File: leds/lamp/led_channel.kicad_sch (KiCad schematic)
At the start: 12 parts, among them J2 Conn_02x05_Top_Bottom, U19 MP5048AGU-Z

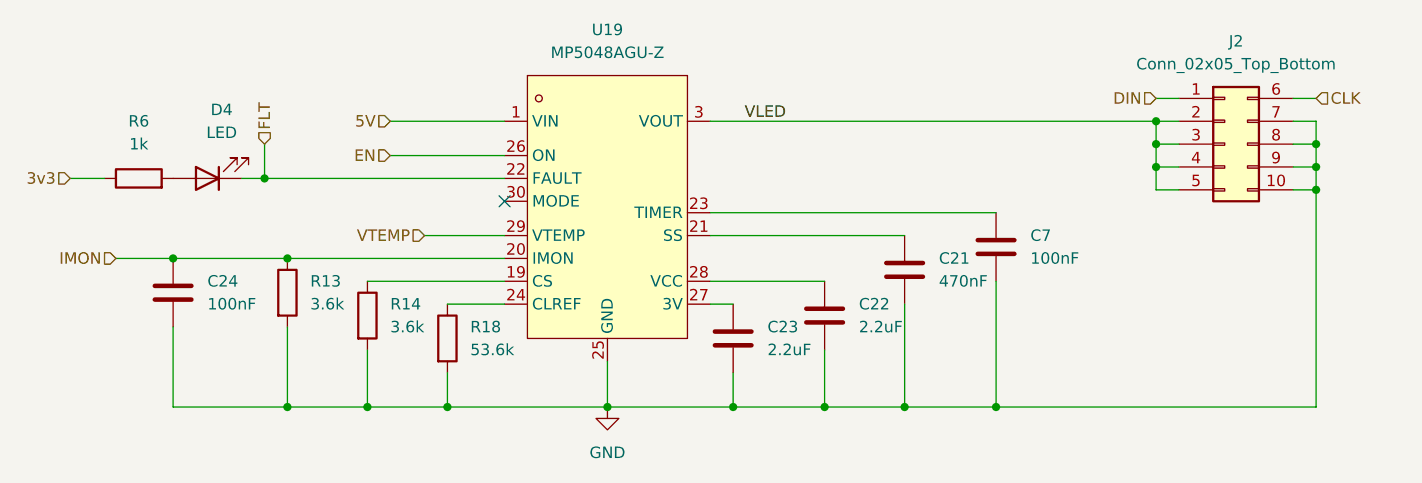
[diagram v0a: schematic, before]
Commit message: WIP: Lamp
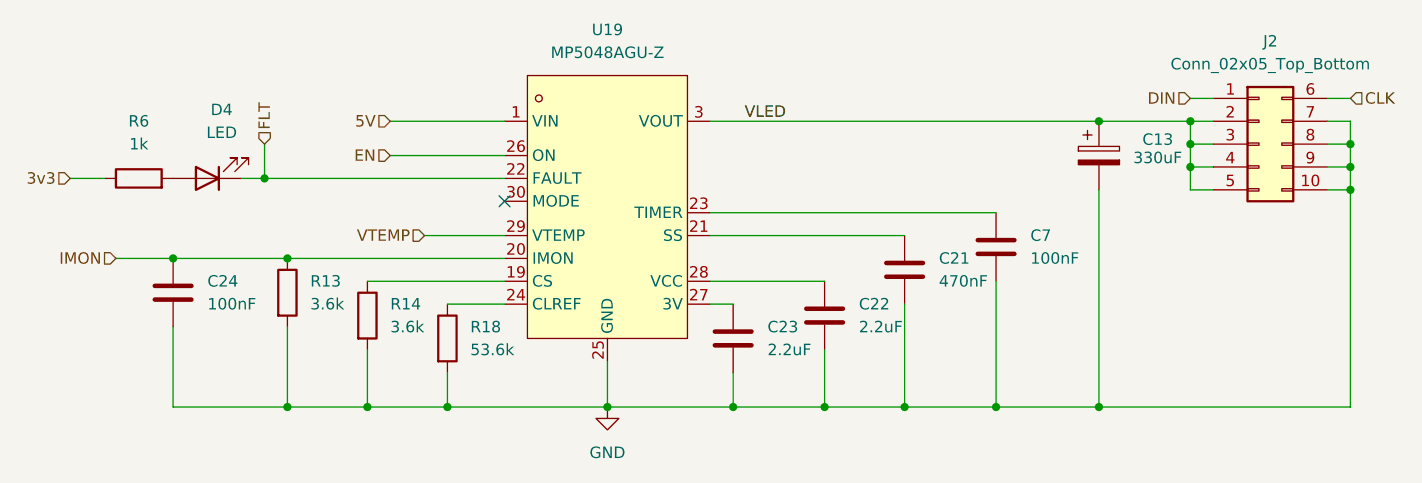
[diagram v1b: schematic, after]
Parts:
- added C13: 330uF, easyeda2kicad:CAP-SMD_L7.3-W4.3-FD, symbol Device:C_Polarized
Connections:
- net GND: now also C13.2
- net VLED: now also C13.1
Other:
- moved on the sheet: J2
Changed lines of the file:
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@@
 	)
 	(junction
-		(at 264.16 74.93)
+		(at 267.97 74.93)
 		(diameter 0)
 		(color 0 0 0 0)
@@
 	)
 	(junction
-		(at 246.38 69.85)
+		(at 250.19 69.85)
 		(diameter 0)
 		(color 0 0 0 0)
@@
 	)
 	(junction
-		(at 246.38 74.93)
+		(at 250.19 74.93)
 		(diameter 0)
 		(color 0 0 0 0)
@@
 	)
 	(junction
-		(at 264.16 72.39)
+		(at 267.97 72.39)
+		(diameter 0)
+		(color 0 0 0 0)
+	)
+	(junction
+		(at 240.03 101.6)
 		(diameter 0)
 		(color 0 0 0 0)
@@
 	)
 	(junction
-		(at 264.16 77.47)
+		(at 267.97 77.47)
 		(diameter 0)
 		(color 0 0 0 0)
@@
 	)
 	(junction
-		(at 246.38 72.39)
+		(at 240.03 69.85)
+		(diameter 0)
+		(color 0 0 0 0)
+	)
+	(junction
+		(at 250.19 72.39)
 		(diameter 0)
 		(color 0 0 0 0)
@@
 	(wire
 		(pts
-			(xy 264.16 74.93) (xy 264.16 77.47)
+			(xy 267.97 74.93) (xy 267.97 77.47)
 		)
 		(stroke
@@
 	(wire
 		(pts
+			(xy 240.03 69.85) (xy 250.19 69.85)
+		)
+		(stroke
+			(width 0)
+			(type default)
+		)
+	)
+	(wire
+		(pts
 			(xy 209.55 101.6) (xy 199.39 101.6)
 		)
@@
 	(wire
 		(pts
-			(xy 264.16 69.85) (xy 264.16 72.39)
+			(xy 267.97 69.85) (xy 267.97 72.39)
 		)
 		(stroke
@@
 	(wire
 		(pts
-			(xy 261.62 67.31) (xy 264.16 67.31)
+			(xy 265.43 67.31) (xy 267.97 67.31)
 		)
 		(stroke
@@
 	(wire
 		(pts
+			(xy 196.85 69.85) (xy 240.03 69.85)
+		)
+		(stroke
+			(width 0)
+			(type default)
+		)
+	)
+	(wire
+		(pts
 			(xy 125.73 76.2) (xy 129.54 76.2)
 		)
@@
 	(wire
 		(pts
+			(xy 240.03 101.6) (xy 267.97 101.6)
+		)
+		(stroke
+			(width 0)
+			(type default)
+		)
+	)
+	(wire
+		(pts
 			(xy 196.85 90.17) (xy 199.39 90.17)
 		)
@@
 	(wire
 		(pts
-			(xy 261.62 72.39) (xy 264.16 72.39)
+			(xy 265.43 72.39) (xy 267.97 72.39)
 		)
 		(stroke
@@
 	(wire
 		(pts
-			(xy 261.62 77.47) (xy 264.16 77.47)
+			(xy 265.43 77.47) (xy 267.97 77.47)
 		)
 		(stroke
@@
 	(wire
 		(pts
-			(xy 248.92 74.93) (xy 246.38 74.93)
+			(xy 252.73 74.93) (xy 250.19 74.93)
 		)
 		(stroke
@@
 	(wire
 		(pts
-			(xy 246.38 77.47) (xy 246.38 74.93)
+			(xy 250.19 77.47) (xy 250.19 74.93)
 		)
 		(stroke
@@
 	(wire
 		(pts
-			(xy 261.62 74.93) (xy 264.16 74.93)
-		)
-		(stroke
-			(width 0)
-			(type default)
-		)
-	)
-	(wire
-		(pts
-			(xy 264.16 77.47) (xy 264.16 101.6)
-		)
-		(stroke
-			(width 0)
-			(type default)
-		)
-	)
-	(wire
-		(pts
-			(xy 264.16 101.6) (xy 228.6 101.6)
-		)
-		(stroke
-			(width 0)
-			(type default)
-		)
-	)
-	(wire
-		(pts
-			(xy 248.92 72.39) (xy 246.38 72.39)
-		)
-		(stroke
-			(width 0)
-			(type default)
-		)
-	)
-	(wire
-		(pts
-			(xy 248.92 77.47) (xy 246.38 77.47)
+			(xy 265.43 74.93) (xy 267.97 74.93)
+		)
+		(stroke
+			(width 0)
+			(type default)
+		)
+	)
+	(wire
+		(pts
+			(xy 267.97 77.47) (xy 267.97 101.6)
+		)
+		(stroke
+			(width 0)
+			(type default)
+		)
+	)
+	(wire
+		(pts
+			(xy 252.73 72.39) (xy 250.19 72.39)
+		)
+		(stroke
+			(width 0)
+			(type default)
+		)
+	)
+	(wire
+		(pts
+			(xy 252.73 77.47) (xy 250.19 77.47)
 		)
 		(stroke
@@
 	(wire
 		(pts
-			(xy 246.38 72.39) (xy 246.38 69.85)
+			(xy 228.6 101.6) (xy 240.03 101.6)
+		)
+		(stroke
+			(width 0)
+			(type default)
+		)
+	)
+	(wire
+		(pts
+			(xy 250.19 72.39) (xy 250.19 69.85)
 		)
 		(stroke
@@
 	(wire
 		(pts
-			(xy 196.85 69.85) (xy 246.38 69.85)
-		)
-		(stroke
-			(width 0)
-			(type default)
-		)
-	)
-	(wire
-		(pts
 			(xy 147.32 72.39) (xy 147.32 76.2)
 		)
@@
 	(wire
 		(pts
-			(xy 246.38 74.93) (xy 246.38 72.39)
-		)
-		(stroke
-			(width 0)
-			(type default)
-		)
-	)
-	(wire
-		(pts
-			(xy 261.62 69.85) (xy 264.16 69.85)
+			(xy 250.19 74.93) (xy 250.19 72.39)
+		)
+		(stroke
+			(width 0)
+			(type default)
+		)
+	)
+	(wire
+		(pts
+			(xy 265.43 69.85) (xy 267.97 69.85)
 		)
 		(stroke
@@
 	(wire
 		(pts
-			(xy 246.38 67.31) (xy 248.92 67.31)
-		)
-		(stroke
-			(width 0)
-			(type default)
-		)
-	)
-	(wire
-		(pts
-			(xy 246.38 69.85) (xy 248.92 69.85)
+			(xy 250.19 67.31) (xy 252.73 67.31)
+		)
+		(stroke
+			(width 0)
+			(type default)
+		)
+	)
+	(wire
+		(pts
+			(xy 250.19 69.85) (xy 252.73 69.85)
 		)
 		(stroke
@@
 	(wire
 		(pts
-			(xy 264.16 72.39) (xy 264.16 74.93)
+			(xy 240.03 77.47) (xy 240.03 101.6)
+		)
+		(stroke
+			(width 0)
+			(type default)
+		)
+	)
+	(wire
+		(pts
+			(xy 267.97 72.39) (xy 267.97 74.93)
 		)
 		(stroke
@@
 	(hierarchical_label "DIN"
 		(shape input)
-		(at 246.38 67.31 180)
+		(at 250.19 67.31 180)
 		(effects
 			(font
@@
 	(hierarchical_label "CLK"
 		(shape input)
-		(at 264.16 67.31 0)
+		(at 267.97 67.31 0)
 		(effects
 			(font
@@
 	(symbol
 		(lib_id "Connector_Generic:Conn_02x05_Top_Bottom")
-		(at 254 72.39 0)
+		(at 257.81 72.39 0)
 		(unit 1)
 		(exclude_from_sim no)
@@
 		(fields_autoplaced yes)
 		(property "Reference" "J2"
-			(at 255.27 60.96 0)
+			(at 259.08 60.96 0)
 			(effects
 				(font
@@
 		)
 		(property "Value" "Conn_02x05_Top_Bottom"
-			(at 255.27 63.5 0)
+			(at 259.08 63.5 0)
 			(effects
 				(font
@@
 		)
 		(property "Footprint" "Connector_Molex:Molex_Nano-Fit_105310-xx10_2x05_P2.50mm_Vertical"
-			(at 254 72.39 0)
+			(at 257.81 72.39 0)
 			(effects
 				(font
@@
 		)
 		(property "Datasheet" "~"
-			(at 254 72.39 0)
+			(at 257.81 72.39 0)
 			(effects
 				(font
@@
 		)
 		(property "Description" "Generic connector, double row, 02x05, top/bottom pin numbering scheme (row 1: 1...pins_per_row, row2: pins_per_row+1 ... num_pins), script generated (kicad-library-utils/schlib/autogen/connector/)"
-			(at 254 72.39 0)
+			(at 257.81 72.39 0)
 			(effects
 				(font
@@
 		)
 		(property "LCSC Part" "C561763"
-			(at 254 72.39 0)
+			(at 257.81 72.39 0)
 			(effects
 				(font
@@
 					(unit 1)
 				)
+			)
+		)
+	)
+	(symbol
+		(lib_id "Device:C_Polarized")
+		(at 240.03 73.66 0)
+		(unit 1)
+		(exclude_from_sim no)
+		(in_bom yes)
+		(on_board yes)
+		(dnp no)
+		(property "Reference" "C13"
+			(at 244.856 71.882 0)
+			(effects
+				(font
+					(size 1.27 1.27)
+				)
+				(justify left)
+			)
+		)
+		(property "Value" "330uF"
+			(at 243.84 73.914 0)
+			(effects
+				(font
+					(size 1.27 1.27)
+				)
+				(justify left)
+			)
+		)
+		(property "Footprint" "easyeda2kicad:CAP-SMD_L7.3-W4.3-FD"
+			(at 240.9952 77.47 0)
+			(effects
+				(font
+					(size 1.27 1.27)
+				)
+				(hide yes)
+			)
+		)
+		(property "Datasheet" "~"
+			(at 240.03 73.66 0)
+			(effects
+				(font
+					(size 1.27 1.27)
+				)
+				(hide yes)
+			)
+		)
+		(property "Description" "Polarized capacitor"
+			(at 240.03 73.66 0)
+			(effects
+				(font
+					(size 1.27 1.27)
+				)
+				(hide yes)
+			)
+		)
+		(property "LCSC Part" "C2159214"
+			(at 240.03 83.82 0)
+			(effects
+				(font
+					(size 1.27 1.27)
+				)
+				(hide yes)
+			)
+		)
+		(property "Label" ""
+			(at 240.03 73.66 0)
+			(effects
+				(font
+					(size 1.27 1.27)
+				)
+				(hide yes)
+			)
+		)
+		(pin "1"
+		)
+		(pin "2"
+		)
+		(instances
+			(project "lamp"
+				(path "/48ddfdd8-68fa-4e63-aa18-bc113cdf8cfa/f2bbebe1-7e19-419b-a0b6-59692ffc8a76"
+					(reference "C13")
+					(unit 1)
+				)
